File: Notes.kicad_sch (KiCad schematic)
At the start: 0 parts

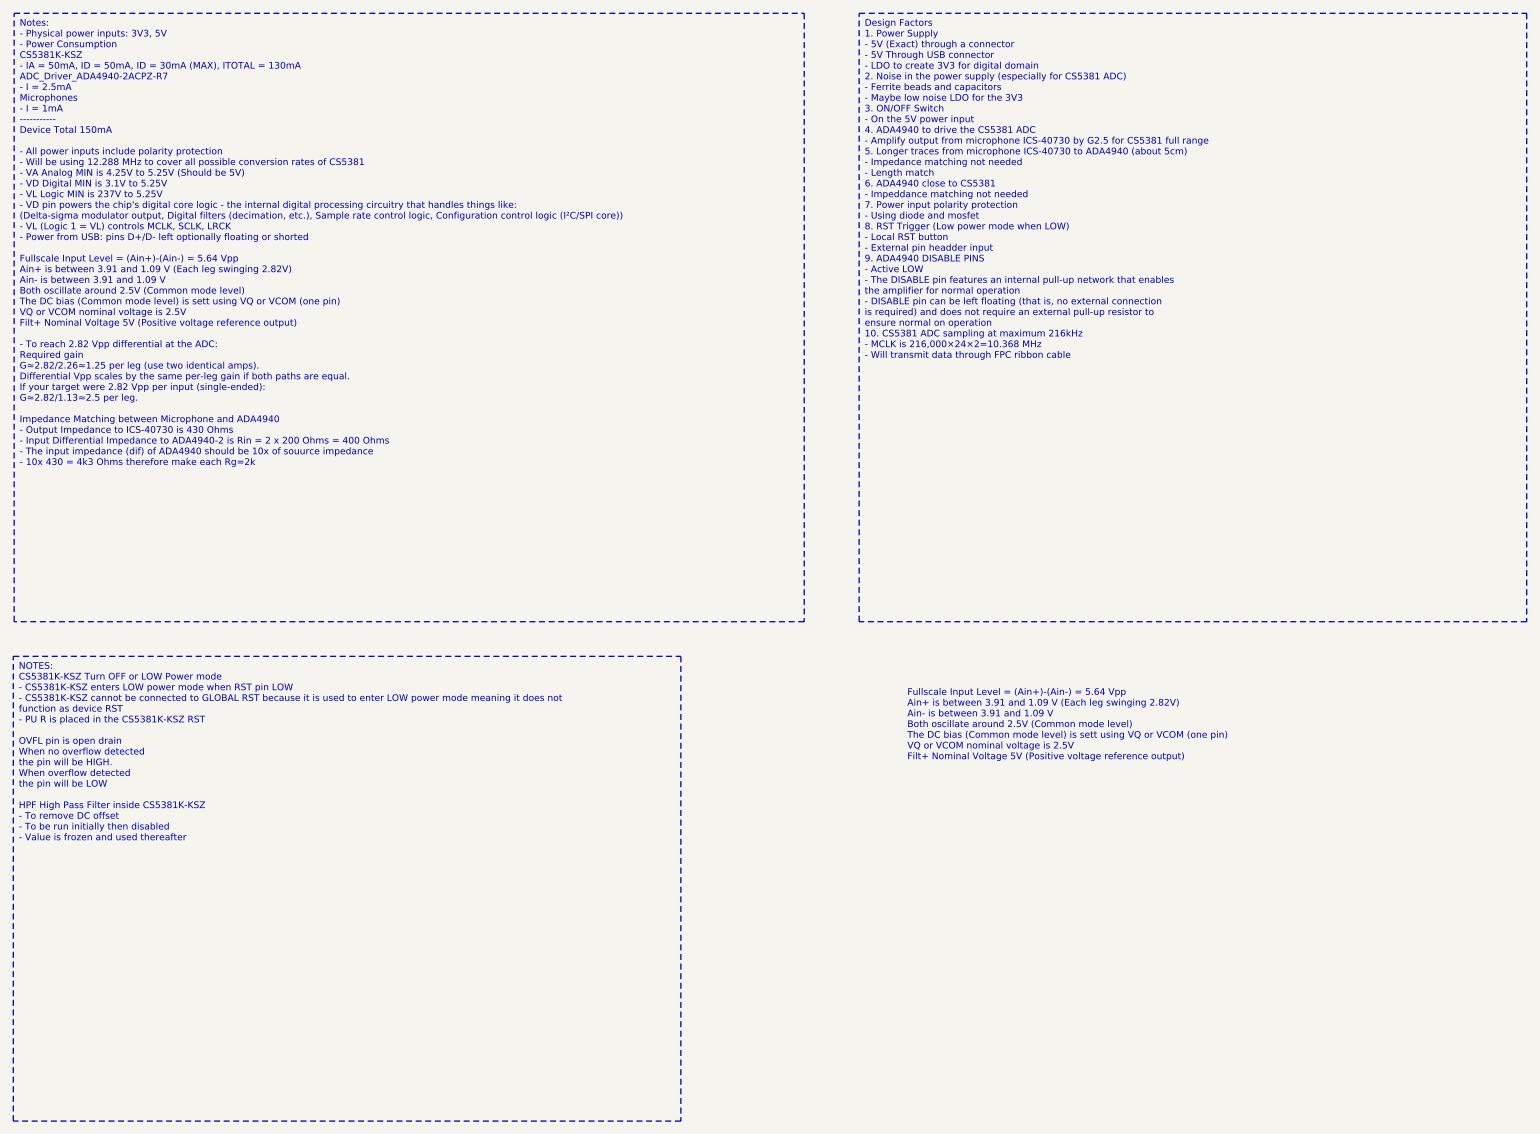
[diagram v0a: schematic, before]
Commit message: Update
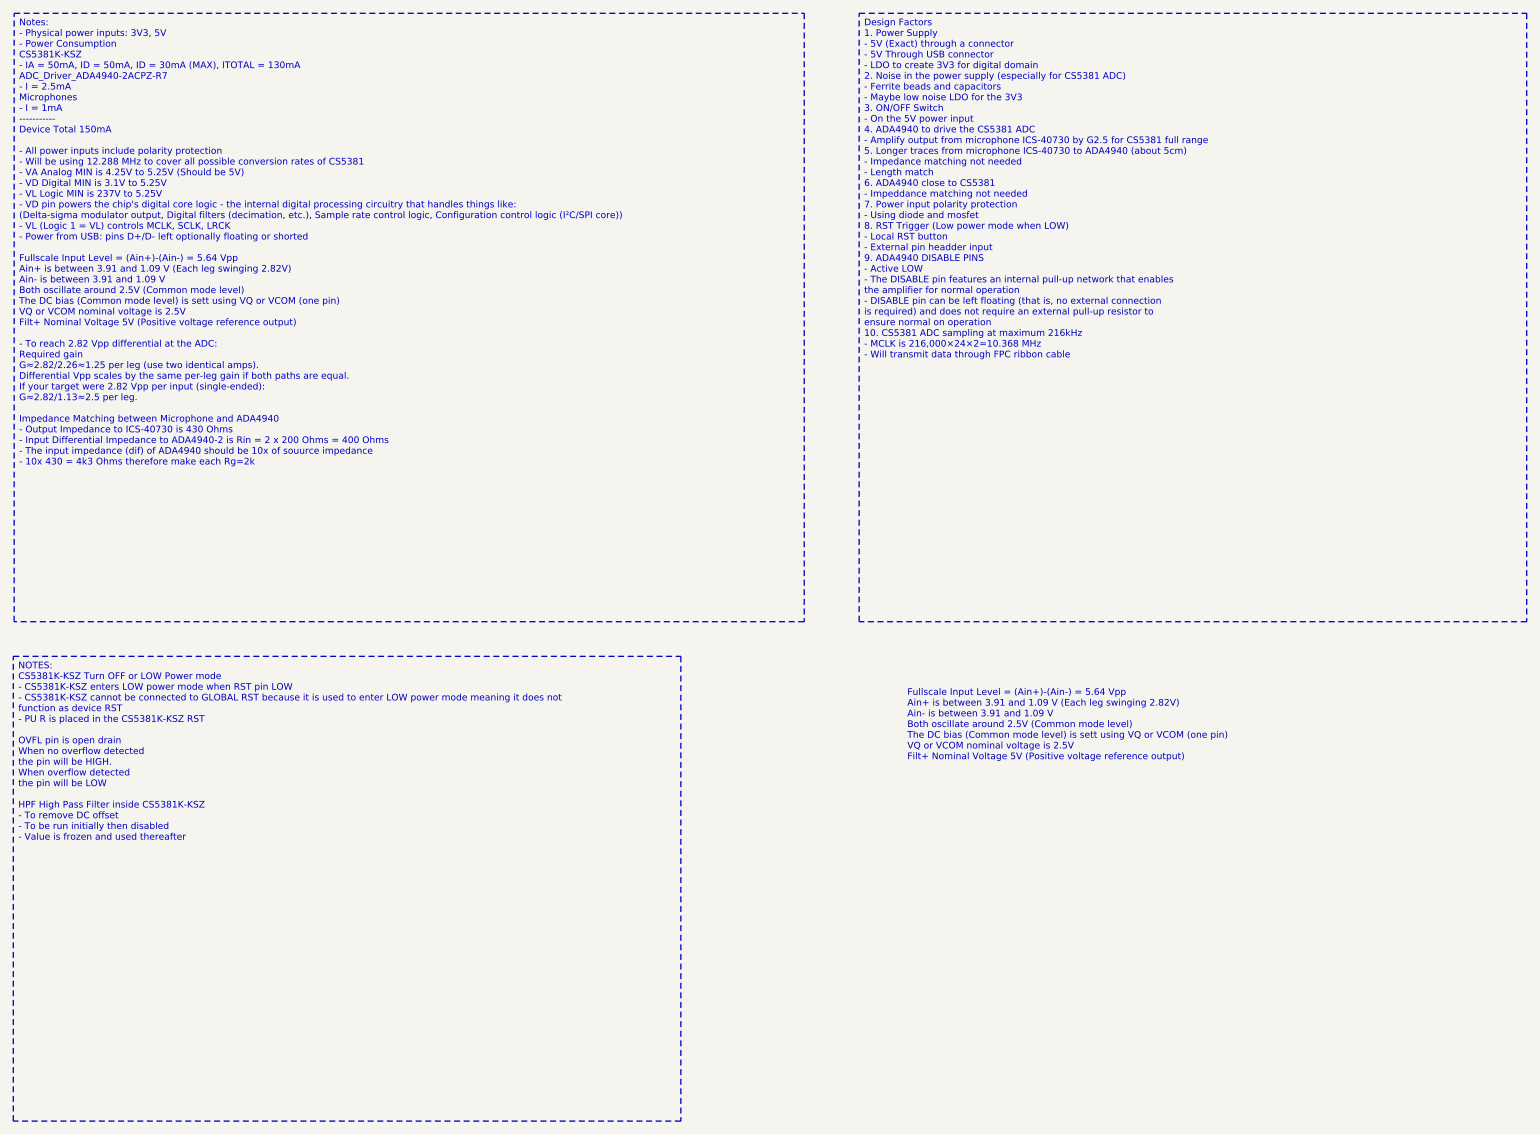
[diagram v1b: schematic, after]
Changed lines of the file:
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@@
 (kicad_sch
-	(version 20231120)
+	(version 20260306)
 	(generator "eeschema")
-	(generator_version "8.0")
+	(generator_version "10.0")
 	(paper "USLetter")
+	(text "Fullscale Input Level = (Ain+)-(Ain-) = 5.64 Vpp\nAin+ is between 3.91 and 1.09 V (Each leg swinging 2.82V)\nAin- is between 3.91 and 1.09 V\nBoth oscillate around 2.5V (Common mode level)\nThe DC bias (Common mode level) is sett using VQ or VCOM (one pin)\nVQ or VCOM nominal voltage is 2.5V\nFilt+ Nominal Voltage 5V (Positive voltage reference output)"
+		(exclude_from_sim no)
+		(at 160.274 133.096 0)
+		(effects
+			(font
+				(size 1 1)
+			)
+			(justify left)
+		)
+	)
 	(text_box "NOTES:\nCS5381K-KSZ Turn OFF or LOW Power mode\n- CS5381K-KSZ enters LOW power mode when RST pin LOW\n- CS5381K-KSZ cannot be connected to GLOBAL RST because it is used to enter LOW power mode meaning it does not function as device RST\n- PU R is placed in the CS5381K-KSZ RST\n\nOVFL pin is open drain\nWhen no overflow detected\nthe pin will be HIGH.\nWhen overflow detected\nthe pin will be LOW\n\nHPF High Pass Filter inside CS5381K-KSZ\n- To remove DC offset\n- To be run initially then disabled\n- Value is frozen and used thereafter "
 		(exclude_from_sim no)
 		(at 25.908 122.682 0)
 		(size 100.33 69.85)
+		(margins 0.75 0.75 0.75 0.75)
 		(stroke
 			(width 0)
@@
 		(at 26.035 26.035 0)
 		(size 118.745 91.44)
+		(margins 0.75 0.75 0.75 0.75)
 		(stroke
 			(width 0)
@@
 		(at 153.035 26.035 0)
 		(size 100.33 91.44)
+		(margins 0.75 0.75 0.75 0.75)
 		(stroke
 			(width 0)
@@
 		)
 	)
-	(text "Fullscale Input Level = (Ain+)-(Ain-) = 5.64 Vpp\nAin+ is between 3.91 and 1.09 V (Each leg swinging 2.82V)\nAin- is between 3.91 and 1.09 V\nBoth oscillate around 2.5V (Common mode level)\nThe DC bias (Common mode level) is sett using VQ or VCOM (one pin)\nVQ or VCOM nominal voltage is 2.5V\nFilt+ Nominal Voltage 5V (Positive voltage reference output)"
-		(exclude_from_sim no)
-		(at 160.274 133.096 0)
-		(effects
-			(font
-				(size 1 1)
-			)
-			(justify left)
-		)
-	)
